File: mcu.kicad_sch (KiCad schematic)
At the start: 7 parts, among them Q5 2N7002, U6 ESP32-C6-MINI-1

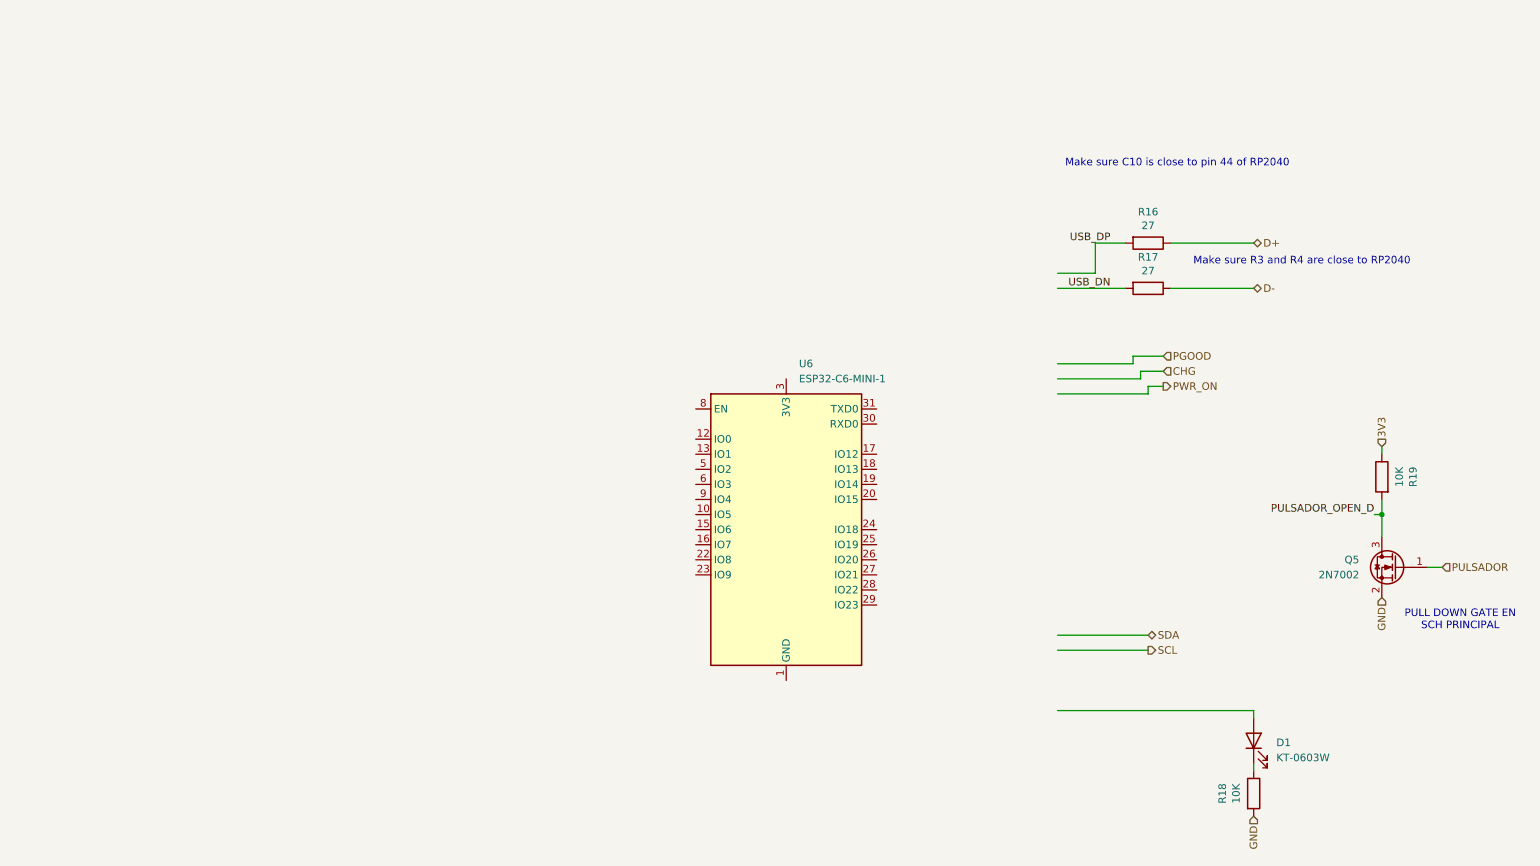
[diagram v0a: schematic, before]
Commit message: Avance de sch
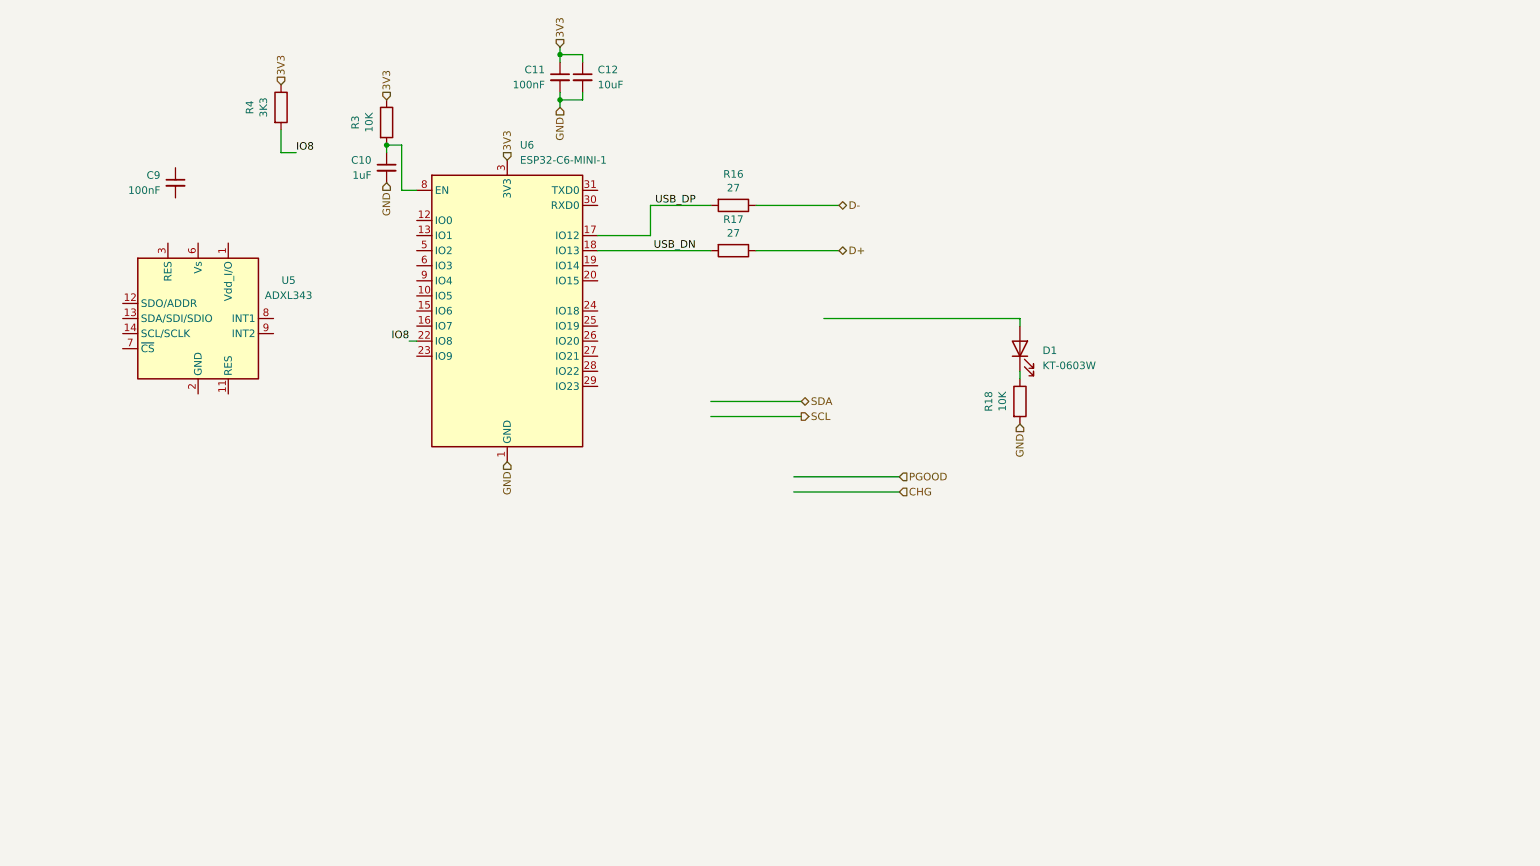
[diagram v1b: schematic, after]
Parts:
- removed Q5: 2N7002, Package_TO_SOT_SMD:SOT-23, symbol Transistor_FET:2N7002
- removed R19: 10K, Resistor_SMD:R_0402_1005Metric, symbol Device:R
- added C10: 1uF, Capacitor_SMD:C_0402_1005Metric, symbol Device:C_Small
- added C11, C9: 100nF, Capacitor_SMD:C_0402_1005Metric, symbol Device:C_Small
- added C12: 10uF, TNG_Passives:C_0603, symbol TNG_Passives:C_10uF_10V_0603
- added R3: 10K, Resistor_SMD:R_0402_1005Metric, symbol Device:R
- added R4: 3K3, Resistor_SMD:R_0402_1005Metric, symbol Device:R
- added U5: ADXL343, Package_LGA:LGA-14_3x5mm_P0.8mm_LayoutBorder1x6y, symbol Sensor_Motion:ADXL343
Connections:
- net 3V3: now also U6.3 (3V3), C11.1, C12.1, R3.1, R4.1
- net D+: now also R17.1; no longer R16.1
- net D-: now also R16.1; no longer R17.1
- net GND: now also U6.1 (GND), U6.11 (GND), U6.14 (GND), U6.2 (GND), U6.36 (GND), U6.37 (GND), U6.38 (GND), U6.39 (GND), U6.40 (GND), U6.41 (GND), U6.42 (GND), U6.43 (GND), U6.44 (GND), U6.45 (GND), U6.46 (GND), U6.47 (GND), U6.48 (GND), U6.49 (GND), U6.50 (GND), U6.51 (GND), U6.52 (GND), U6.53 (GND), C10.2, C11.2, C12.2
- net USB_DN: now also U6.18 (IO13)
- net USB_DP: now also U6.17 (IO12)
- net IO8: now reaches U6.22 (IO8)
- net IO8: now also R4.2
- net at U6.8 (EN): now also C10.1, R3.2
- new net: U5.2 (GND), U5.4 (GND), U5.5 (GND)
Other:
- note removed: "Make sure C10 is close to pin 44 of RP2040"
- note removed: "Make sure R3 and R4 are close to RP2040"
- note removed: "PULL DOWN GATE EN SCH PRINCIPAL"
- moved on the sheet: D1, R16, R17, R18, U6

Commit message: Casi que placa lista
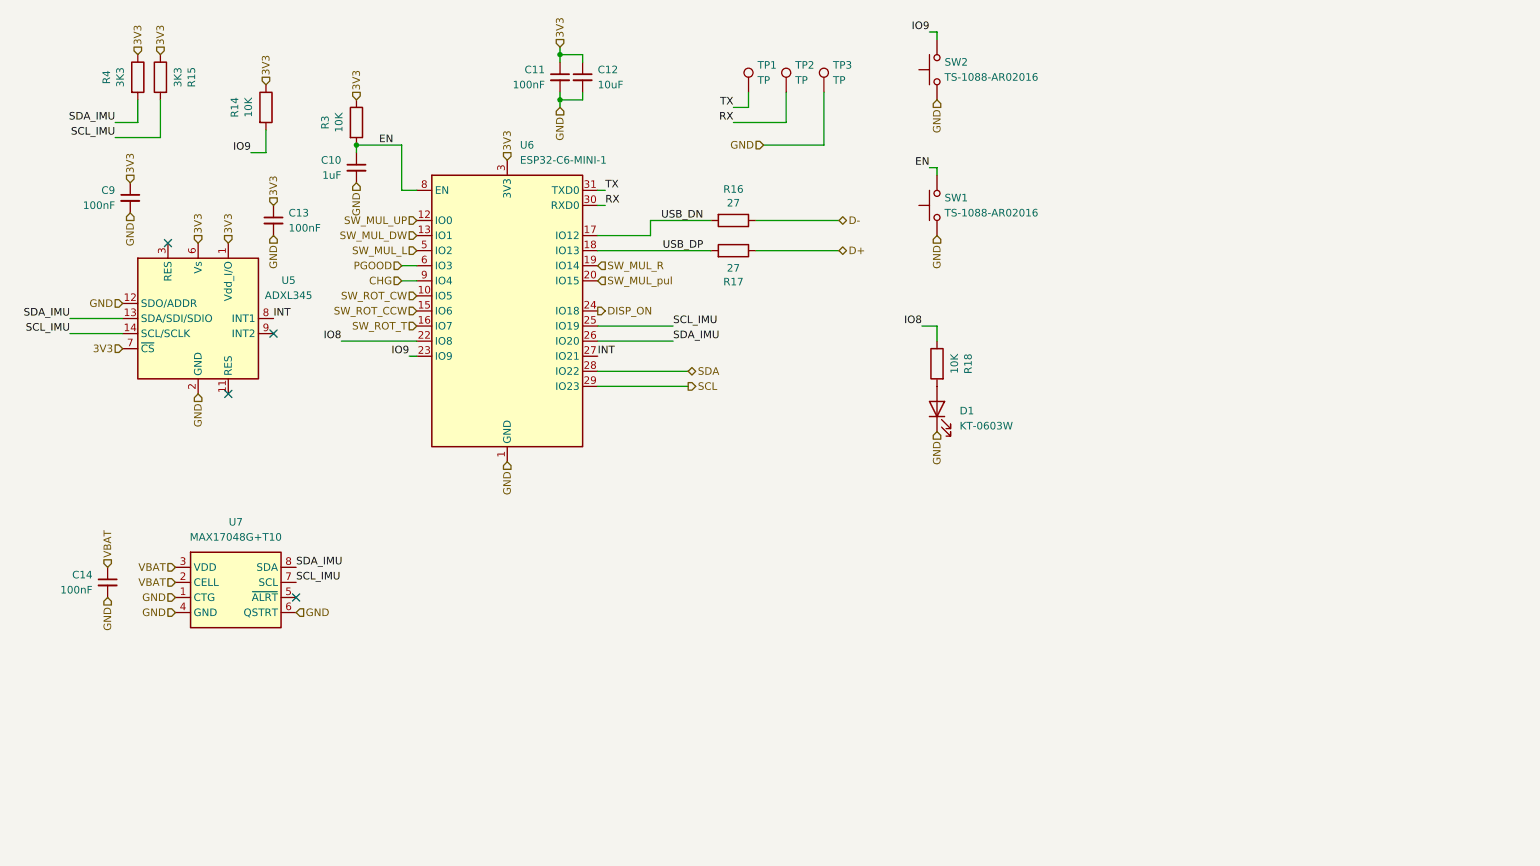
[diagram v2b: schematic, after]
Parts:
- added C13, C14: 100nF, Capacitor_SMD:C_0402_1005Metric, symbol Device:C_Small
- added R14: 10K, Resistor_SMD:R_0402_1005Metric, symbol Device:R
- added R15: 3K3, Resistor_SMD:R_0402_1005Metric, symbol Device:R
- added SW1, SW2: TS-1088-AR02016, footprints:TS-1088-AR02016, symbol Switch:SW_Omron_B3FS
- added TP1, TP2, TP3: TP, TestPoint:TestPoint_Pad_D1.5mm, symbol Connector:TestPoint
- added U7: MAX17048G+T10, Package_DFN_QFN:TDFN-8-1EP_2x2mm_P0.5mm_EP0.8x1.2mm, symbol TNG_ICs:MAX17048G+T10
- U5: value ADXL343 -> ADXL345
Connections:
- net 3V3: now also C9.1, U5.1 (Vdd_I/O), U5.6 (Vs), U5.7 (~{CS}), C13.1, R14.1, R15.1
- net CHG: now also U6.9 (IO4)
- net GND: now also C9.2, D1.1 (K), U5.12 (SDO/ADDR), U5.2 (GND), U5.4 (GND), U5.5 (GND), C13.2, C14.2, SW1.1, SW2.1, TP3.1, U7.1 (CTG), U7.4 (GND), U7.6 (QSTRT), U7.9 (EP); no longer R18.2
- net IO8: now also R18.1; no longer R4.2
- net PGOOD: now also U6.6 (IO3)
- net SCL: now also U6.29 (IO23)
- net SDA: now also U6.28 (IO22)
- net USB_DN: now also R16.2, U6.17 (IO12); no longer R17.2, U6.18 (IO13)
- net USB_DP: now also R17.2, U6.18 (IO13); no longer R16.2, U6.17 (IO12)
- net at D1.2 (A): now also R18.2
- net SDA_IMU: now reaches U5.13 (SDA/SDI/SDIO)
- net SDA_IMU: now also R4.2, U6.26 (IO20), U7.8 (SDA)
- net SCL_IMU: now reaches U5.14 (SCL/SCLK)
- net SCL_IMU: now also U6.25 (IO19), R15.2, U7.7 (SCL)
- net INT: now reaches U5.8 (INT1)
- net INT: now also U6.27 (IO21)
- net SW_ROT_CW: now reaches U6.10 (IO5)
- net SW_MUL_UP: now reaches U6.12 (IO0)
- net SW_MUL_DW: now reaches U6.13 (IO1)
- net SW_ROT_CCW: now reaches U6.15 (IO6)
- net SW_ROT_T: now reaches U6.16 (IO7)
- net SW_MUL_R: now reaches U6.19 (IO14)
- net SW_MUL_pul: now reaches U6.20 (IO15)
- net IO9: now reaches U6.23 (IO9)
- net IO9: now also R14.2, SW2.2
- net DISP_ON: now reaches U6.24 (IO18)
- net RX: now reaches U6.30 (RXD0)
- net RX: now also TP2.1
- net TX: now reaches U6.31 (TXD0)
- net TX: now also TP1.1
- net SW_MUL_L: now reaches U6.5 (IO2)
- net EN: now reaches C10.1, R3.2, U6.8 (EN)
- net EN: now also SW1.2
- new net VBAT: C14.1, U7.2 (CELL), U7.3 (VDD)
- no-connect marks 0 -> 4
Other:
- moved on the sheet: C10, C9, D1, R16, R18, R3
